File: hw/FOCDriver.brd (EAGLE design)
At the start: 99.1 x 62.2 mm, 118 parts, among them Q1 BC817, Q2 BC817, Q3 BC817, Q4 BC817, Q5 BC817, Q6 BC817, U1 SN74LVC2G17, U10 LMV321SQ3T2G, U11 LMV321SQ3T2G, U2 AO4606, U3 BA7805FP, U4 SN74LVC2G17, U5 AO4606, U6 SN74LVC2G17, U7 AO4606, U8 LMV321SQ3T2G, U9 LMV321SQ3T2G

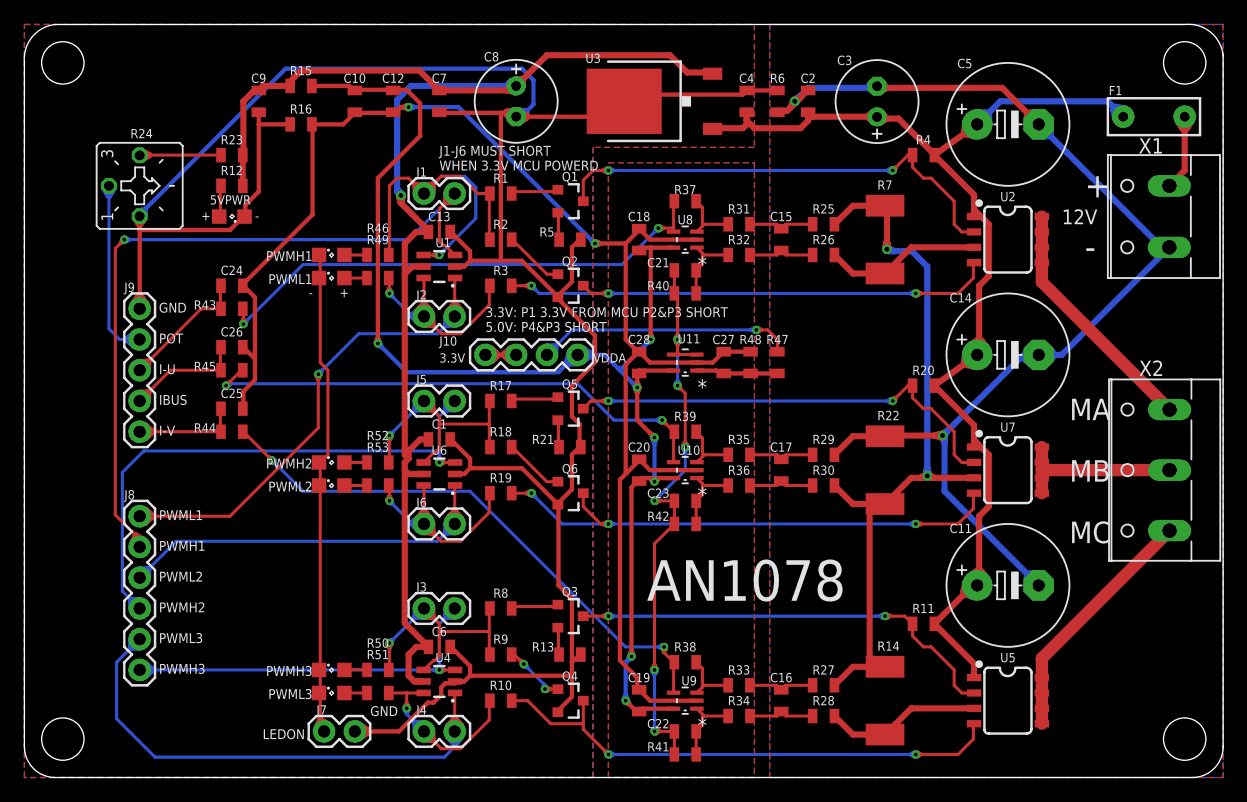
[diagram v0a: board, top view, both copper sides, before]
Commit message: fix error
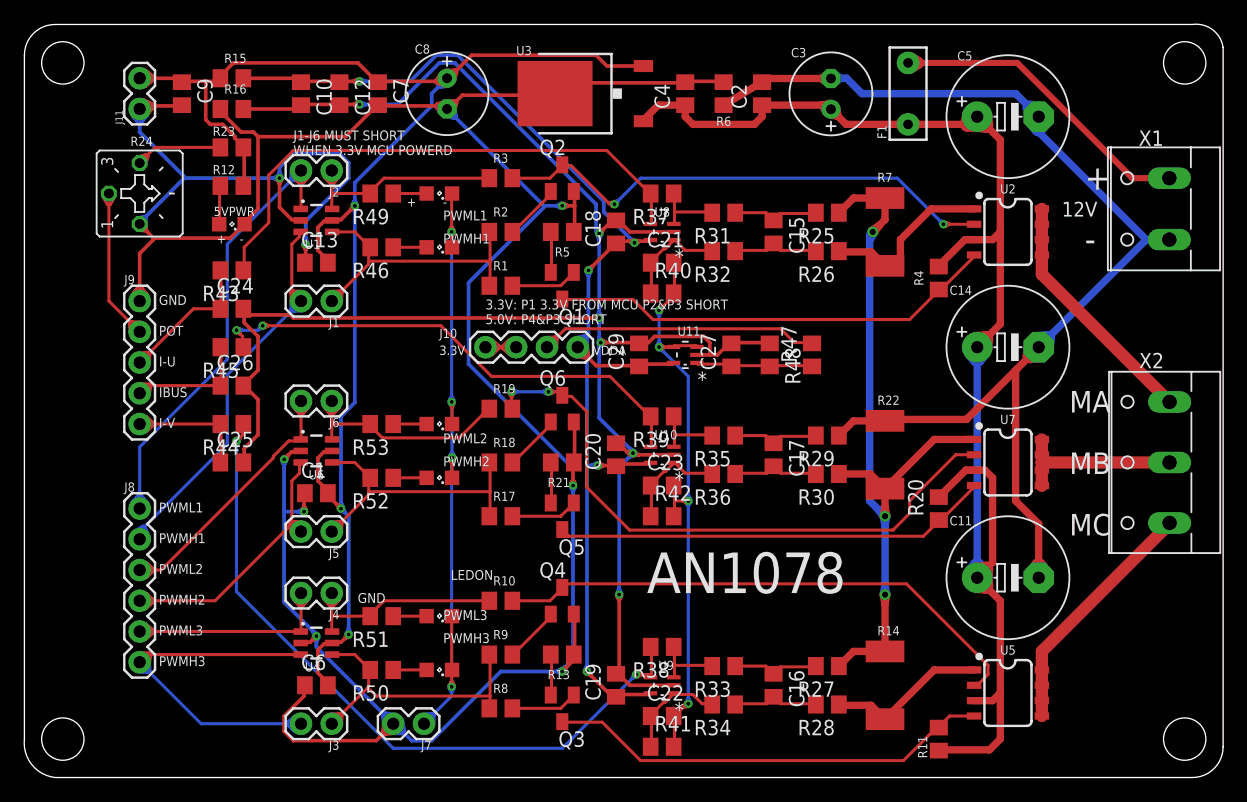
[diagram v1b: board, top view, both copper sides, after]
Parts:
- removed C28: 0.1uF, SparkFun-Capacitors:0805
- added C29: 0.1u, rcl:C0805
- added J11: (no value), SparkFun-Connectors:1X02
- C1, C10, C12, C13, C6, C7, C9: value 0.1uF -> 100n; device SparkFun-Capacitors:0805 -> rcl:C0805
- C15, C16, C17, C21, C22, C23: value 56pF -> 56p; device SparkFun-Capacitors:0805 -> rcl:C0805
- C18, C19, C2, C20, C27, C4: value 0.1uF -> 0.1u; device SparkFun-Capacitors:0805 -> rcl:C0805
- C24, C25, C26: value 1nF -> 1n; device SparkFun-Capacitors:0805 -> rcl:C0805
- Q1, Q2, Q3, Q4, Q5, Q6: device SparkFun-DiscreteSemi:SOT23-3 -> transistor-npn:SOT23-BEC
- R1, R10, R11, R12, R13, R17, R18, R19, R2, R20, R21, R23, R3, R4, R46, R49, R5, R50, R51, R52, R53, R8, R9: device SparkFun-Resistors:0805 -> rcl:R0805
- R15: value 1R -> 0; device SparkFun-Resistors:0805 -> rcl:R0805
- R16, R6: value 0R -> 0; device SparkFun-Resistors:0805 -> rcl:R0805
- R25, R26, R27, R28, R29, R30, R31, R32, R33, R34, R35, R36, R43, R44, R45: value 1K 1% -> 1K; device SparkFun-Resistors:0805 -> rcl:R0805
- R37, R38, R39, R40, R41, R42, R47, R48: value 20K 1% -> 20K; device SparkFun-Resistors:0805 -> rcl:R0805
- moved F1 20.4 mm to (73.0, 56.5), turned to 270 degrees
- moved J2 17.5 mm to (22.9, 50.2), turned to 0 degrees
- moved J4 17.1 mm to (22.9, 15.2), turned to 0 degrees
- moved J5 16.7 mm to (22.9, 20.3), turned to 0 degrees
- moved J6 16.3 mm to (22.9, 31.1), turned to 0 degrees
- moved J3 15.9 mm to (22.9, 4.45), turned to 0 degrees
- moved J1 15.5 mm to (22.9, 39.4), turned to 0 degrees
- moved LED3 11.3 mm to (34.3, 48.3), turned to 180 degrees
- moved C1 11.1 mm to (24.1, 23.5)
- moved LED5 10.9 mm to (34.3, 13.3), turned to 180 degrees
- moved U1 10.9 mm to (24.1, 46.0), turned to 90 degrees
- moved C6 10.6 mm to (24.1, 7.62)
- moved U4 10.6 mm to (24.1, 11.1), turned to 90 degrees
- moved C13 10.5 mm to (24.1, 42.5)
- moved U6 10.3 mm to (24.1, 27.0), turned to 90 degrees
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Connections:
- net 5V: now also C1.2, C13.2, C6.2, J11.2, R23.1; no longer C1.1, C13.1, C6.1, R23.2
- net AGND: now also C29.2; no longer C28.2
- net DGND: now also C1.1, C13.1, C6.1, J11.1, Q2.E, Q4.E, Q6.E; no longer C1.2, C13.2, C6.2, Q2.2, Q4.2, Q6.2
- net ICOM: now also U7.1; no longer U7.3
- net IU: now also U2.1; no longer U2.3
- net IV: now also U5.1; no longer U5.3
- net N$10: now also Q1.C, U2.4; no longer Q1.3, U2.2
- net N$15: now also C21.1; no longer C21.2
- net N$20: now also C22.1; no longer C22.2
- net N$25: now also C23.1; no longer C23.2
- net N$28: now also Q5.E; no longer Q5.2
- net N$3: now also Q6.C, U7.2; no longer Q6.3, U7.4
- net N$30: now also Q1.B; no longer Q1.1
- net N$32: now also Q2.B; no longer Q2.1
- net N$39: now also Q3.B; no longer Q3.1
- net N$4: now also R23.2; no longer R23.1
- net N$40: now also Q1.E; no longer Q1.2
- net N$41: now also Q4.B; no longer Q4.1
- net N$42: now also Q5.B; no longer Q5.1
- net N$43: now also Q3.E; no longer Q3.2
- net N$44: now also Q6.B; no longer Q6.1
- net N$6: now also Q5.C, U7.4; no longer Q5.3, U7.2
- net N$7: now also Q4.C, U5.2; no longer Q4.3, U5.4
- net N$8: now also Q3.C, U5.4; no longer Q3.3, U5.2
- net N$9: now also Q2.C, U2.2; no longer Q2.3, U2.4
- net VDDA: now also C29.1; no longer C28.1
- net VIN: now also U2.3, U5.3, U7.3; no longer U2.1, U5.1, U7.1
- net VREF: now also C21.2, C22.2, C23.2; no longer C21.1, C22.1, C23.1
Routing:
- net DGND: track 234.5 -> 351.6 mm, vias 0 -> 8
- net VREF: track 176.5 -> 78.2 mm, vias 6 -> 4
- net VDDA: track 206.3 -> 136.6 mm, vias 7 -> 5
- net N$9: track 112.9 -> 51.0 mm, vias 3 -> 2
- net LEDON: track 43.5 -> 104.6 mm, vias 0 -> 5
- net N$3: track 115.1 -> 64.6 mm, vias 3 -> 2
- net AGND: track 155.3 -> 200.6 mm, vias 2 -> 6
- net L2: track 74.8 -> 31.0 mm
- net N$8: track 80.5 -> 37.2 mm, vias 2 -> 0
- net H2: track 83.7 -> 42.0 mm, vias 1 -> 0
- net H1: track 79.5 -> 40.2 mm, vias 1 -> 0
- net N$10: track 75.5 -> 37.2 mm, vias 2 -> 0
- net H3: track 72.8 -> 34.7 mm, vias 1 -> 0
- net N$6: track 73.7 -> 36.3 mm, vias 2 -> 0
- net N$7: track 78.7 -> 45.0 mm, vias 2 -> 0
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- removed copper zone on layer 1, net AGND
- removed copper zone on layer 16, net AGND
- removed copper zone on layer 1, net DGND
- removed copper zone on layer 16, net DGND
- removed copper zone on layer 1, net GND
- removed copper zone on layer 16, net GND
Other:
- board size 99.1 x 62.2 mm -> 99.1 x 62.3 mm
